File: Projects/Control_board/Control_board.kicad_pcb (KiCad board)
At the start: 2 copper layers, 99.5 x 100.4 mm, 83 parts, among them IC1 VN7050ASTR, IC2 PCA9615DPJ, IC3 PSSI2021SAY,115, J1 66200621022, J10 43045-0401, J11 Conn_01x04, J12 Conn_01x04, J13 Conn_01x01_Female, J2 66200621022, J3 43045-0200, J4 43045-0200, J5 43045-0401, J6 RJ45, J7 66200621022, J8 Conn_01x02, Q1 Q_NMOS_GSD, Q2 BSS138-Transistor_FET, Q3 BSP76_E6433, Q4 Q_PMOS_GDS, Q5 BSP76_E6433, U1 ESP32-DEVKITC-32D, U2 NCP1117-5.0_TO252, U3 NID35-12_meanwell

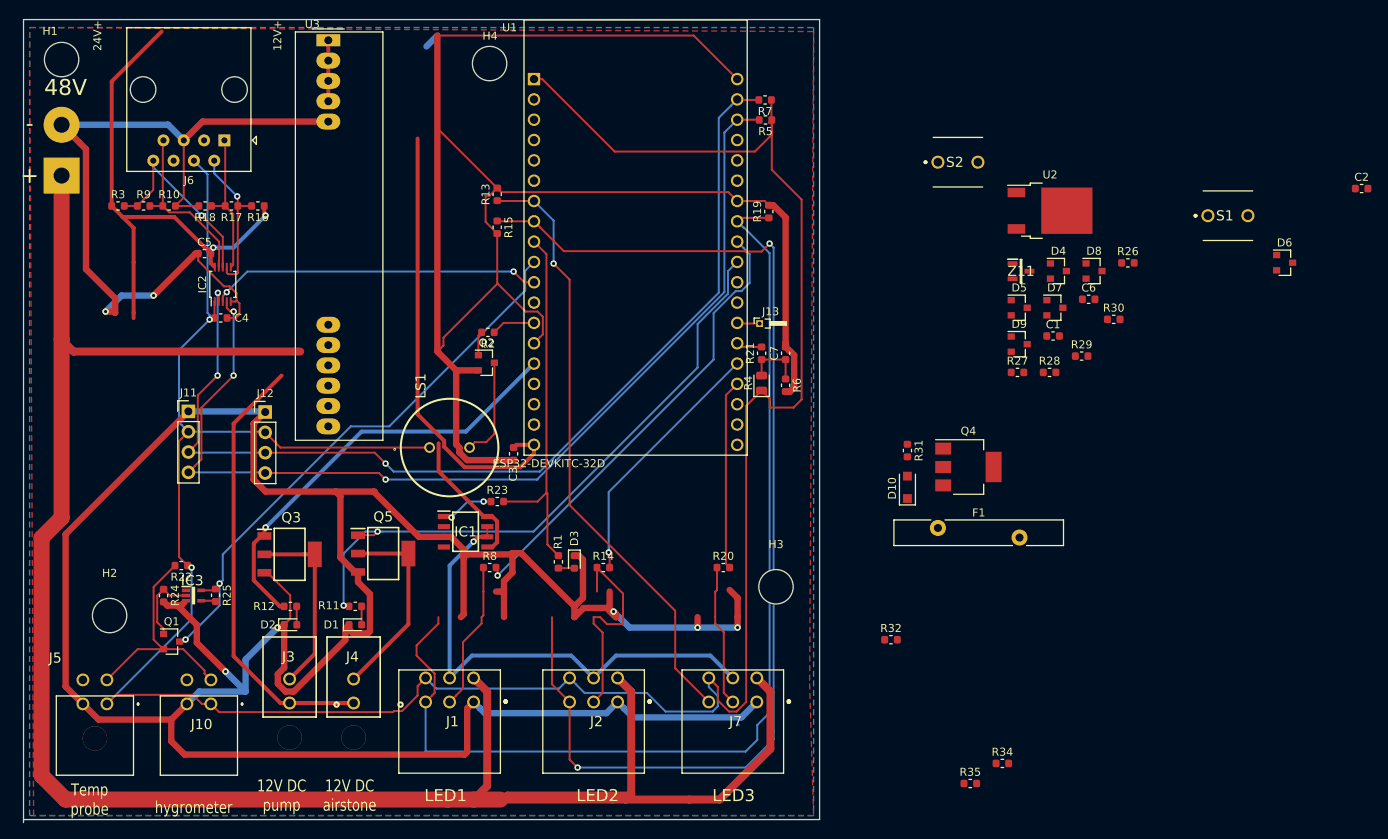
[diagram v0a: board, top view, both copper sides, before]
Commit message: updated PCB
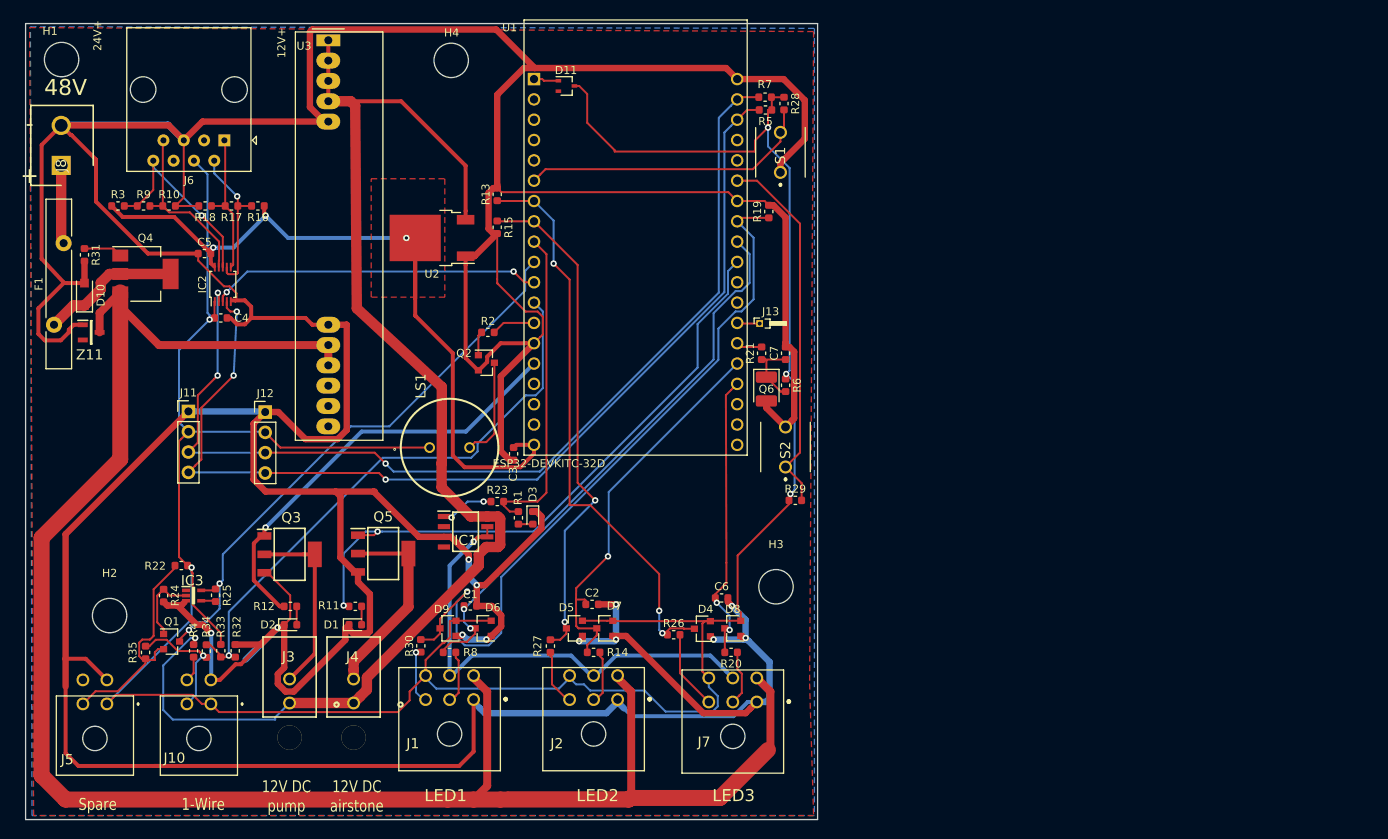
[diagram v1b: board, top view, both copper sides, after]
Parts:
- added D11: BAT54W, Package_TO_SOT_SMD:SOT-323_SC-70, F.Cu at (146.6, 90.8)
- added Q6: Q_Photo_NPN, Diode_SMD:D_1210_3225Metric_Pad1.42x2.65mm_HandSolder, F.Cu at (171.6, 128.7)
- added R33: DNP, Resistor_SMD:R_0603_1608Metric, F.Cu at (105.2, 161.4)
- D4, D5, D6, D7, D8, D9: value BAT54S -> BAT54SLT1G
- J10, J5: value 43045-0401 -> 43045-0401_2
- J8: value Conn_01x02 -> TB003-500-P02BE; footprint Connector_Wire:SolderWirePad_1x02_P7.62mm_Drill2mm -> SamacSys_Parts:SHDR2W100P0X500_1X2_1000X780X1030P
- R4: value LDR03 -> DNP; footprint LED_SMD:LED_0805_2012Metric -> Resistor_SMD:R_0603_1608Metric
- moved Z11 116.5 mm to (87.2, 121.6)
- moved F1 113.4 mm to (82.5, 120.7), turned to 90 degrees
- moved D6 110.1 mm to (136.2, 158.6), turned to 180 degrees
- moved C2 109.3 mm to (149.8, 155.6)
- moved R31 105.7 mm to (86.4, 111.9)
- moved D10 105.7 mm to (86.4, 116.8)
- moved Q4 105.7 mm to (94.0, 114.3)
- moved R35 104.4 mm to (94.0, 161.6), turned to 270 degrees
- moved R34 100.5 mm to (101.6, 161.4), turned to 270 degrees
- moved R30 95.7 mm to (128.4, 160.8), turned to 90 degrees
- moved R32 83.8 mm to (103.4, 161.4), turned to 270 degrees
- moved C1 80.3 mm to (134.6, 155.8)
- moved D9 79.8 mm to (131.8, 158.6), turned to 180 degrees
- moved R4 78.5 mm to (100.0, 161.4), turned to 270 degrees
- moved U2 77.3 mm to (129.8, 109.8), turned to 180 degrees
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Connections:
- J10 pad 2: GND -> Net-(J10-Pad2)
- J10 pad 3: Net-(J10-Pad3) -> GND
- J5 pad 2: GND -> Net-(J5-Pad2)
- J5 pad 3: Net-(J5-Pad3) -> GND
- Q1 pad 2: Net-(J5-Pad3) -> Net-(J5-Pad2)
- R22 pad 2: Net-(J5-Pad3) -> Net-(J5-Pad2)
- R34 pad 2: Net-(J10-Pad3) -> Net-(J10-Pad2)
- R35 pad 1: Net-(J10-Pad3) -> Net-(J10-Pad2)
- R35 pad 2: Net-(J5-Pad3) -> Net-(J5-Pad2)
- R4 pad 1: +3V3 -> +12V
- R4 pad 2: Net-(C7-Pad1) -> Net-(J10-Pad4)
- R6 pad 1: Net-(C7-Pad1) -> +3V3
- R6 pad 2: GND -> Net-(C7-Pad1)
- U1 pad 1: +3V3 -> Net-(D11-Pad1)
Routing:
- net /NTC_2: track 144.5 -> 7.19 mm, vias 2 -> 0
- net GND: track 683.1 -> 811.3 mm, vias 7 -> 12
- net /NTC_1: track 132.7 -> 7.31 mm, vias 0 -> 1
- net Net-(D9-Pad3): track 0.00 -> 92.2 mm, vias 0 -> 1
- net +12V: track 80.1 -> 168.5 mm, vias 0 -> 1
- net /Spare: track 0.00 -> 73.3 mm, vias 0 -> 1
- net Net-(D4-Pad3): track 0.00 -> 71.5 mm, vias 0 -> 3
- net /NTC_3: track 76.3 -> 9.89 mm, vias 1 -> 0
- net Net-(D5-Pad3): track 0.00 -> 63.3 mm, vias 0 -> 2
- net Net-(R29-Pad2): track 0.06 -> 46.3 mm
- net Net-(R28-Pad2): track 0.00 -> 37.0 mm
- net Net-(J10-Pad3): track 28.5 -> 0.00 mm
- net Net-(J5-Pad2): track 0.00 -> 28.5 mm
- net +3V3: track 328.4 -> 355.9 mm, vias 2 -> 5
- net +5V: track 121.4 -> 98.9 mm, vias 2 -> 3
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- added copper zone on F.Cu, net +5V
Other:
- board size 99.5 x 100.4 mm -> 99 x 99.5 mm
- net class 48volt: trace_width 1 -> 1.3
- net class Power: trace_width 0.8 -> 0.5
- net class Power_2: trace_width 0.5 -> 1.3
- board text added: "1-Wire"
- board text added: "Spare"
- board text removed: "Temp probe"
- board text removed: "hygrometer"
